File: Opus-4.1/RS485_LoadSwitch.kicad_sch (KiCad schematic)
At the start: 32 parts, among them J1 PWR_IN, J2 RS485, J3 OUT1, J4 OUT2, J5 OUT3, J6 OUT4, J7 SWD, U5 INA181A3, Y1 8MHz

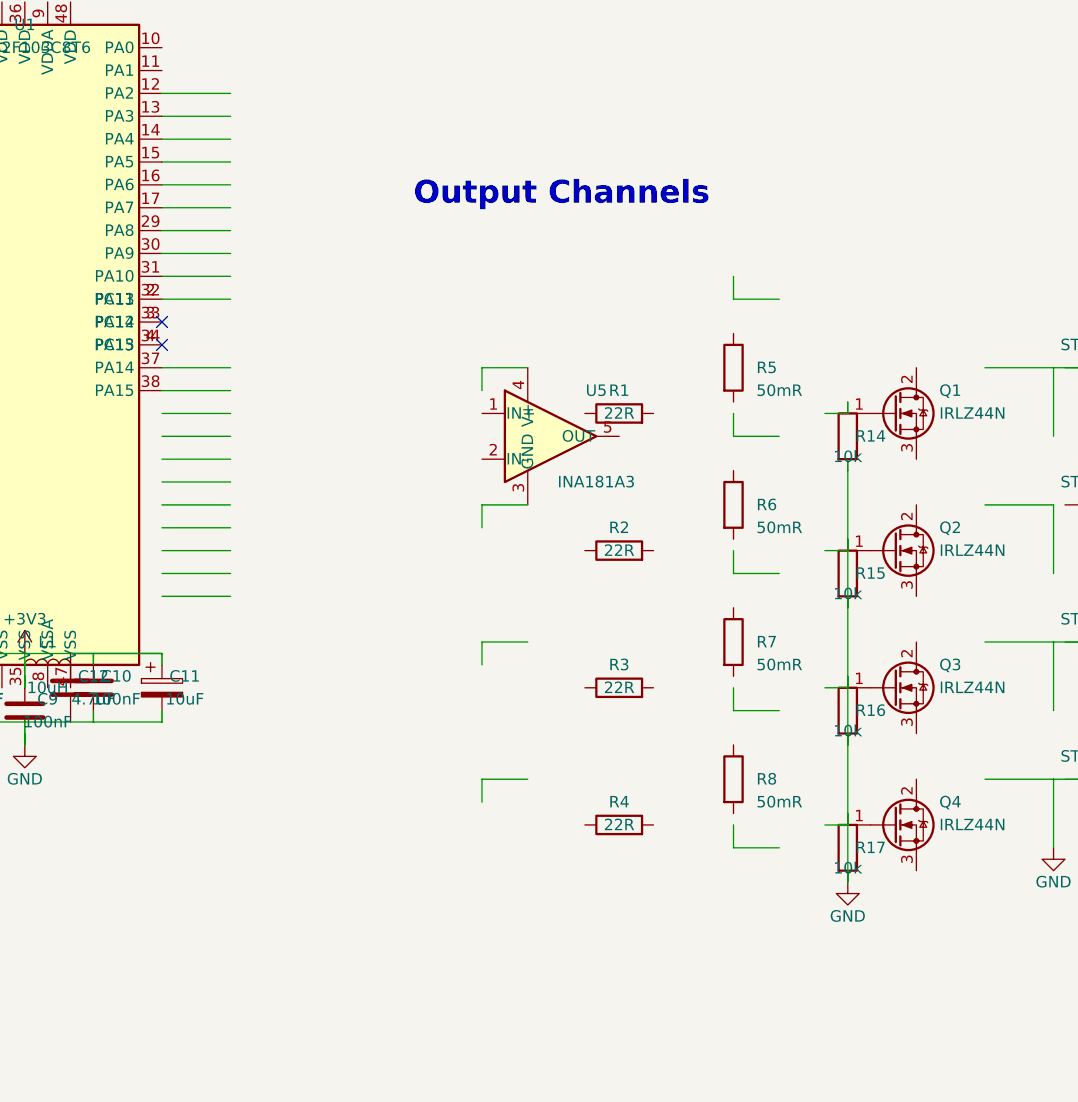
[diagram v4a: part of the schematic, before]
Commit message: Add files via upload
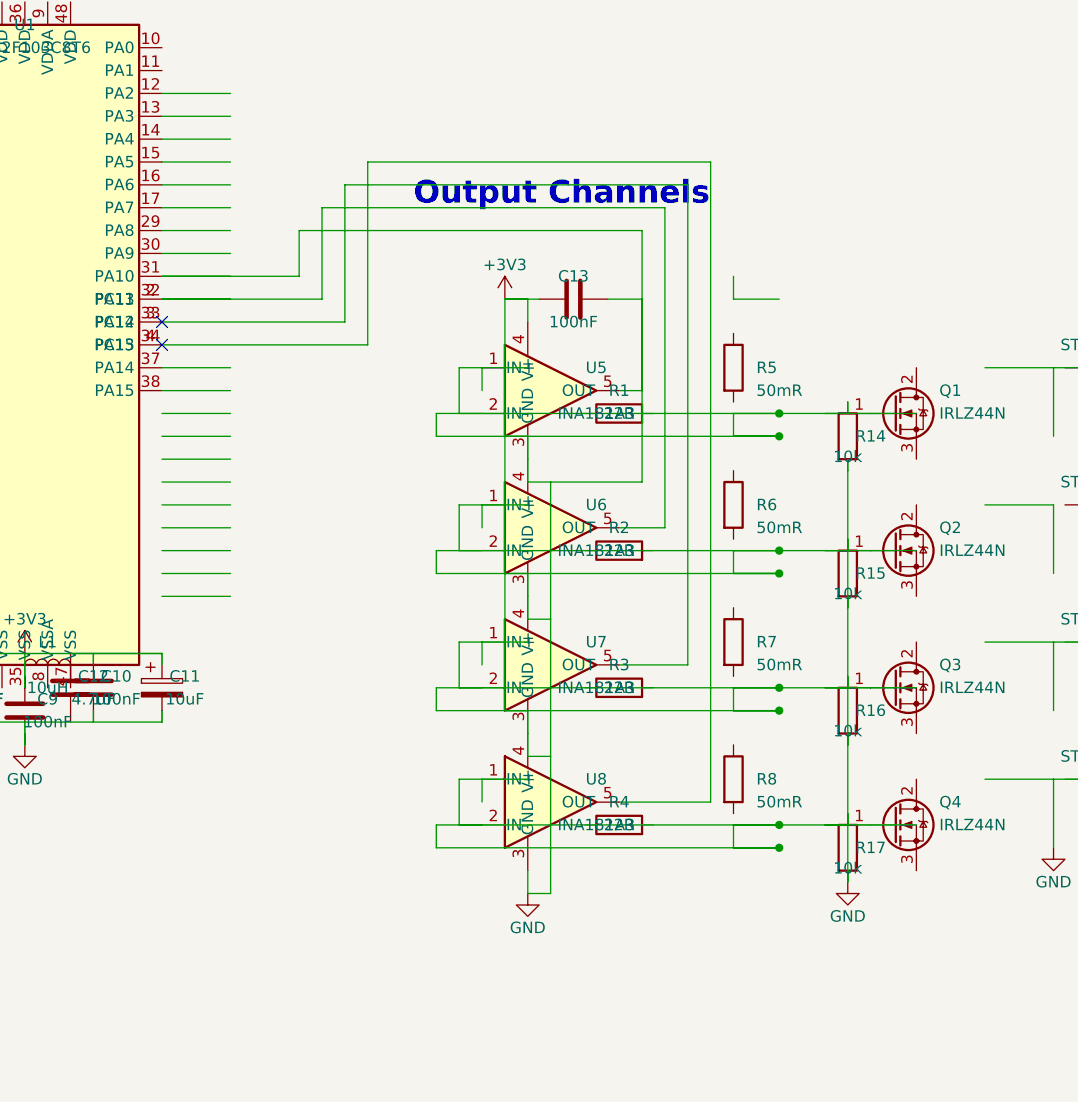
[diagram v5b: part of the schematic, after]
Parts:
- added C13: 100nF, Capacitor_SMD:C_0603_1608Metric, symbol Device:C
- added U6, U7, U8: INA181A3, Package_TO_SOT_SMD:SOT-23-5, symbol Amplifier_Current:INA181
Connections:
- net GND is gone; now on net +3V3: C10.2, C11.2, C8.2, C8.2, C9.2, D6.1 (A1), D7.1 (A1), D8.1 (A1), J1.2 (Pin_2), J2.2 (Pin_2), J3.2 (Pin_2), J4.2 (Pin_2), R14.2, R15.1, R15.2, R16.1, R16.2, R17.1, R17.2
- net +3V3: now also J3.31 (PA10), J7.1 (Pin_1), R14.1, U5.1 (IN+), U5.2 (IN-), U5.3 (GND), U5.4 (V+), U5.5 (OUT), C13.1, C13.2, U6.1 (IN+), U6.2 (IN-), U6.3 (GND), U6.4 (V+), U7.1 (IN+), U7.2 (IN-), U7.3 (GND), U7.4 (V+), U8.1 (IN+), U8.2 (IN-), U8.3 (GND), U8.4 (V+)
- net at J3.2 (Pin_2), J3.32 (PA11): now also U6.5 (OUT)
- net at J3.3 (PC14), J3.33 (PA12): now also U7.5 (OUT)
- net at J3.34 (PA13), J3.4 (PC15): now also U8.5 (OUT)
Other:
- moved on the sheet: U5

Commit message: Add files via upload
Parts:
- added C14: 10nF, Capacitor_SMD:C_0805_2012Metric, symbol Device:C
- added C18: 470uF/25V, Capacitor_THT:CP_Radial_D10.0mm_P5.00mm, symbol Device:CP
- added D10, D11, D12, D9: 15V, Diode_SMD:D_SOD-123, symbol Device:D_Zener
- added R18: 100R, Resistor_SMD:R_0805_2012Metric, symbol Device:R
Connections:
- net +3V3 is gone; now on net +12V: C10.1, C10.2, C11.1, C11.2, C12.1, C13.1, C13.2, C8.1, C8.1, C8.2, C8.2, C9.1, C9.2, D6.1 (A1), D7.1 (A1), D8.1 (A1), J1.2 (Pin_2), J2.2 (Pin_2), J3.2 (Pin_2), J3.31 (PA10), J3.35 (VSS), J4.2 (Pin_2), J7.1 (Pin_1), R14.1, R14.2, R15.1, R15.2, R16.1, R16.2, R17.1, R17.2, U5.1 (IN+), U5.2 (IN-), U5.3 (GND), U5.4 (V+), U5.5 (OUT), U6.1 (IN+), U6.2 (IN-), U6.3 (GND), U6.4 (V+), U7.1 (IN+), U7.2 (IN-), U7.3 (GND), U7.4 (V+), U8.1 (IN+), U8.2 (IN-), U8.3 (GND), U8.4 (V+)
- net +12V: now also D6.3 (S), D7.2 (A2), D7.3 (S), D8.2 (A2), D8.3 (S), J3.1 (Pin_1), J4.1 (Pin_1), J5.1 (Pin_1), J5.2 (Pin_2), J6.1 (Pin_1), J6.2 (Pin_2), J7.2 (Pin_2), J7.3 (Pin_3), C18.1, C18.2
- new net: D6.2 (A2), J4.2 (Pin_2)

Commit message: Add files via upload
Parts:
- added BT1: CR2032, Battery:BatteryHolder_Keystone_3034_1x20mm, symbol Device:Battery_Cell
- added D13: PWR, LED_SMD:LED_0805_2012Metric, symbol Device:LED
- added D14: COMM, LED_SMD:LED_0805_2012Metric, symbol Device:LED
- added J8: SWD, Connector_PinHeader_2.54mm:PinHeader_1x05_P2.54mm_Vertical, symbol Connector:Conn_01x05_Pin
- added R22, R23: 470R, Resistor_SMD:R_0603_1608Metric, symbol Device:R
- added R24: 10k, Resistor_SMD:R_0603_1608Metric, symbol Device:R
- added U1: STM32F103C8T6, Package_QFP:LQFP-48_7x7mm_P0.5mm, symbol MCU_ST_STM32F1:STM32F103C8Tx
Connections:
- net +12V: now also C12.2, U6.5 (OUT), U7.5 (OUT), U8.5 (OUT), Y1.1, U1.12 (PA2), U1.13 (PA3), U1.14 (PA4), U1.15 (PA5), U1.2 (PC13), U1.23 (VSS), U1.3 (PC14), U1.31 (PA10), U1.32 (PA11), U1.33 (PA12), U1.34 (PA13), U1.35 (VSS), U1.4 (PC15), U1.7 (NRST); no longer J3.31 (PA10), J3.35 (VSS)
- net at D6.2 (A2): no longer J4.2 (Pin_2)
- new net: D6.2 (A2), J4.2 (Pin_2)
- new net: C12.1, U1.36 (VDD)
- new net: D13.1 (K), D14.1 (K), U1.18 (PB0), U1.19 (PB1)
- new net: D14.2 (A), R23.2
- new net: D13.2 (A), R22.2
- new net: R22.1, R23.1
- new net: U1.21 (PB10), U1.46 (PB9)
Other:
- moved on the sheet: C19, L1

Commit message: Add files via upload
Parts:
- added C15, C16, C17: 10nF/100V, Capacitor_SMD:C_0805_2012Metric, symbol Device:C
- added C20, C21, C22, C23, C24, C25, C26: 100nF, Capacitor_SMD:C_0603_1608Metric, symbol Device:C
- added D13: SS54, Diode_SMD:D_SMB, symbol Device:D_Schottky
- added D14: STPS3L60, Diode_SMD:D_SMB, symbol Diode:STPS3L60
- added D15, D16: PESD1CAN, Package_TO_SOT_SMD:SOT-23, symbol Device:D_TVS_ALT
- added D17: CH1, LED_SMD:LED_0603_1608Metric, symbol Device:LED
- added F1: 5A, Fuse:Fuse_1206_3216Metric, symbol Device:Fuse
- added L2: 33uH/5A, Inductor_SMD:L_12x12mm_H8mm, symbol Device:L
- added L3: 100uH CM, Inductor_SMD:L_CommonMode_Wuerth_WE-SL2, symbol Device:L_Coupled
- added R19, R20, R21: 100R, Resistor_SMD:R_0805_2012Metric, symbol Device:R
- added R25, R26, R27, R28, R29: 1k, Resistor_SMD:R_0603_1608Metric, symbol Device:R
- added TP1: 12V, TestPoint:TestPoint_Pad_D1.5mm, symbol Connector:TestPoint
- added TP2: 5V, TestPoint:TestPoint_Pad_D1.5mm, symbol Connector:TestPoint
- added TP3: 3V3, TestPoint:TestPoint_Pad_D1.5mm, symbol Connector:TestPoint
- added TP4: GND, TestPoint:TestPoint_Pad_D1.5mm, symbol Connector:TestPoint
- U5, U6, U7, U8: value INA181A3 -> INA181A1
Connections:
- net at D6.2 (A2): no longer J4.2 (Pin_2)
- new net: D6.2 (A2), J4.2 (Pin_2)
- new net: C20.2, C23.1
